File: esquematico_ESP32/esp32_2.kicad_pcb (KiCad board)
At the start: 2 copper layers, 79.6 x 93.5 mm, 39 parts, among them J2 Conn_RFID1, J3 Conn_RFID2, J4 USB_A, J5 Conn_screen, J6 Conn_01x04_Female, J7 Jack-DC, Q1 BSS138, Q2 BSS138, SW1 SW_Push, SW2 Enable, U1 ESP32-WROOM-32, U2 LM1117-3.3, U3 LM2596S-5

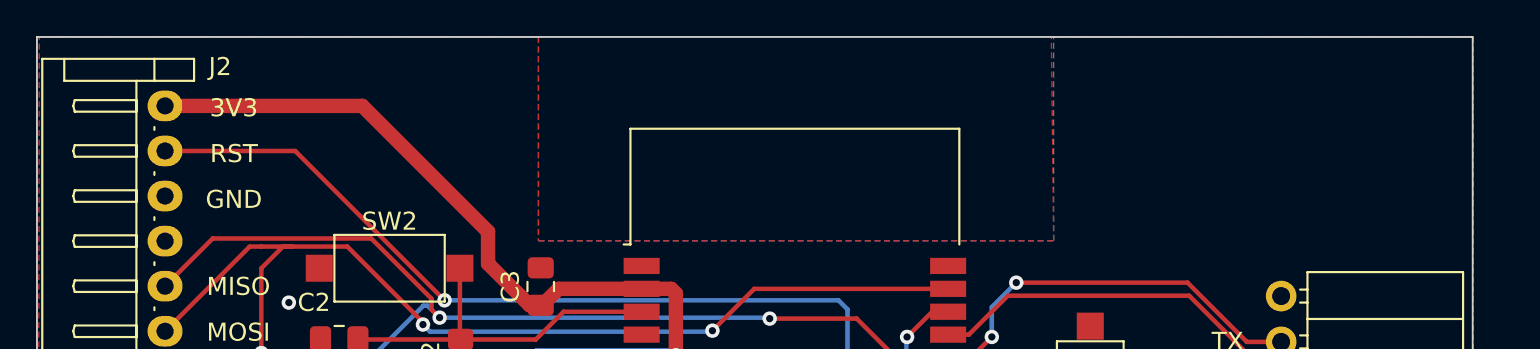
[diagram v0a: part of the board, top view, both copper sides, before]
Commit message: diseño listo
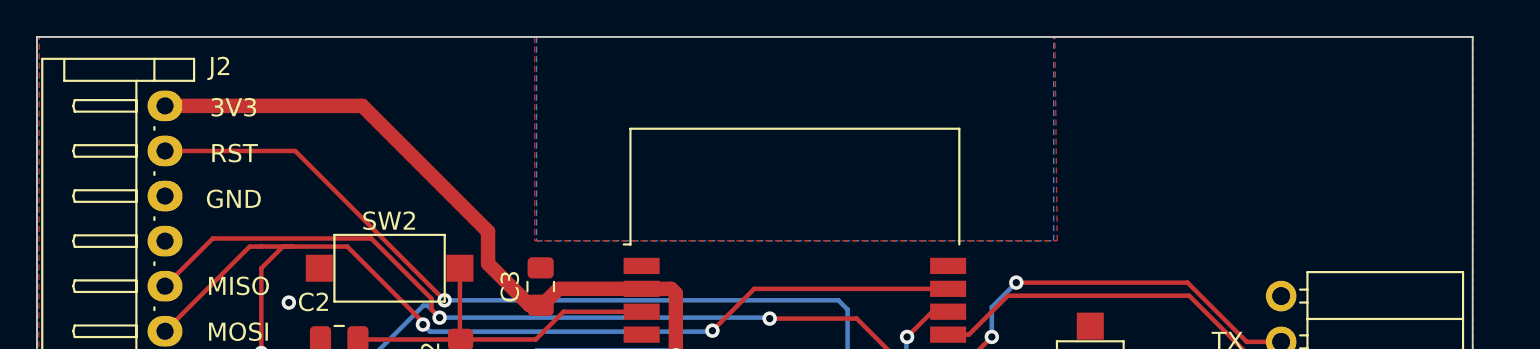
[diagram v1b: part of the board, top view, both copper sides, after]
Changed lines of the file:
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@@
   (segment (start 167.894 100.711) (end 167.894 93.628) (width 1) (layer "B.Cu") (net 46))
   (segment (start 167.894 93.628) (end 166.546 92.28) (width 1) (layer "B.Cu") (net 46))
-  (zone (net 0) (net_name "") (layers F&B.Cu) (hatch edge 0.508)
-    (connect_pads (clearance 0))
-    (min_thickness 0.254)
-    (keepout (tracks not_allowed) (vias not_allowed) (pads not_allowed ) (copperpour not_allowed) (footprints not_allowed))
-    (fill (thermal_gap 0.508) (thermal_bridge_width 0.508))
-    (polygon
-      (pts
-        (xy 186.563 39.243)
-        (xy 158.115 39.243)
-        (xy 158.115 28.067)
-        (xy 186.563 28.067)
-      )
-    )
-  )
   (zone (net 4) (net_name "GND") (layer "F.Cu") (hatch edge 0.508)
     (connect_pads (clearance 0.508))
@@
     (polygon
       (pts
-        (xy 158.115 39.37)
-        (xy 186.69 39.37)
-        (xy 186.563 28.067)
+        (xy 157.9118 39.37)
+        (xy 186.888609 39.367768)
+        (xy 186.761609 28.064768)
         (xy 209.931 28.067)
         (xy 209.931 121.539)
         (xy 130.302 121.412)
         (xy 130.429 28.067)
-        (xy 158.115 28.067)
+        (xy 157.9118 28.067)
       )
     )
@@
     (polygon
       (pts
-        (xy 158.115 39.37)
+        (xy 158.0134 39.37)
         (xy 186.69 39.37)
         (xy 186.69 28.067)
@@
         (xy 130.302 121.539)
         (xy 130.302 28.067)
-        (xy 158.115 28.067)
+        (xy 158.0134 28.067)
       )
     )
